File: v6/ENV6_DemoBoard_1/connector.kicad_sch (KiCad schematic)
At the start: 9 parts, among them J501 Conn_02x16_Odd_Even, J502 Conn_02x04_Odd_Even, J503 Conn_02x16_Odd_Even, J504 Conn_02x04_Odd_Even, J505 Conn_02x16_Odd_Even

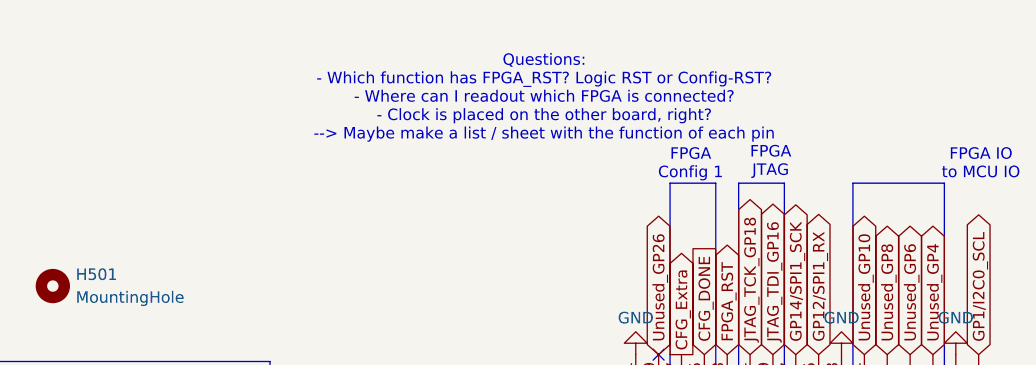
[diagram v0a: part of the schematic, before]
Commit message: updated Baseboard
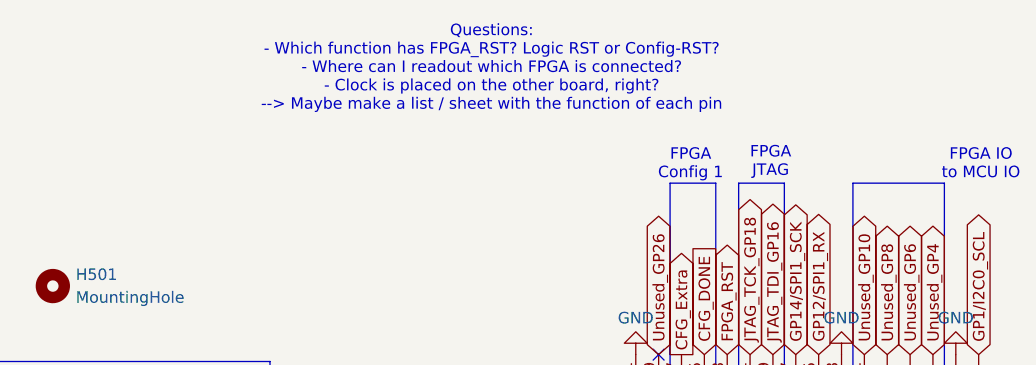
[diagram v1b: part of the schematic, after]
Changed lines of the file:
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@@
 	(text "Questions:\n- Which function has FPGA_RST? Logic RST or Config-RST?\n- Where can I readout which FPGA is connected?\n- Clock is placed on the other board, right?\n--> Maybe make a list / sheet with the function of each pin"
 		(exclude_from_sim no)
-		(at 124.46 17.272 0)
+		(at 118.618 13.97 0)
 		(effects
 			(font
